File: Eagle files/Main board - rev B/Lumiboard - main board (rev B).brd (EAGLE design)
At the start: 49.7 x 42.2 mm, 29 parts, among them IC1 MCP1700, IC2 ULN2003AD, U1 ATMEGA328, U2 DX_BT_MODULE, Y1 8Mhz

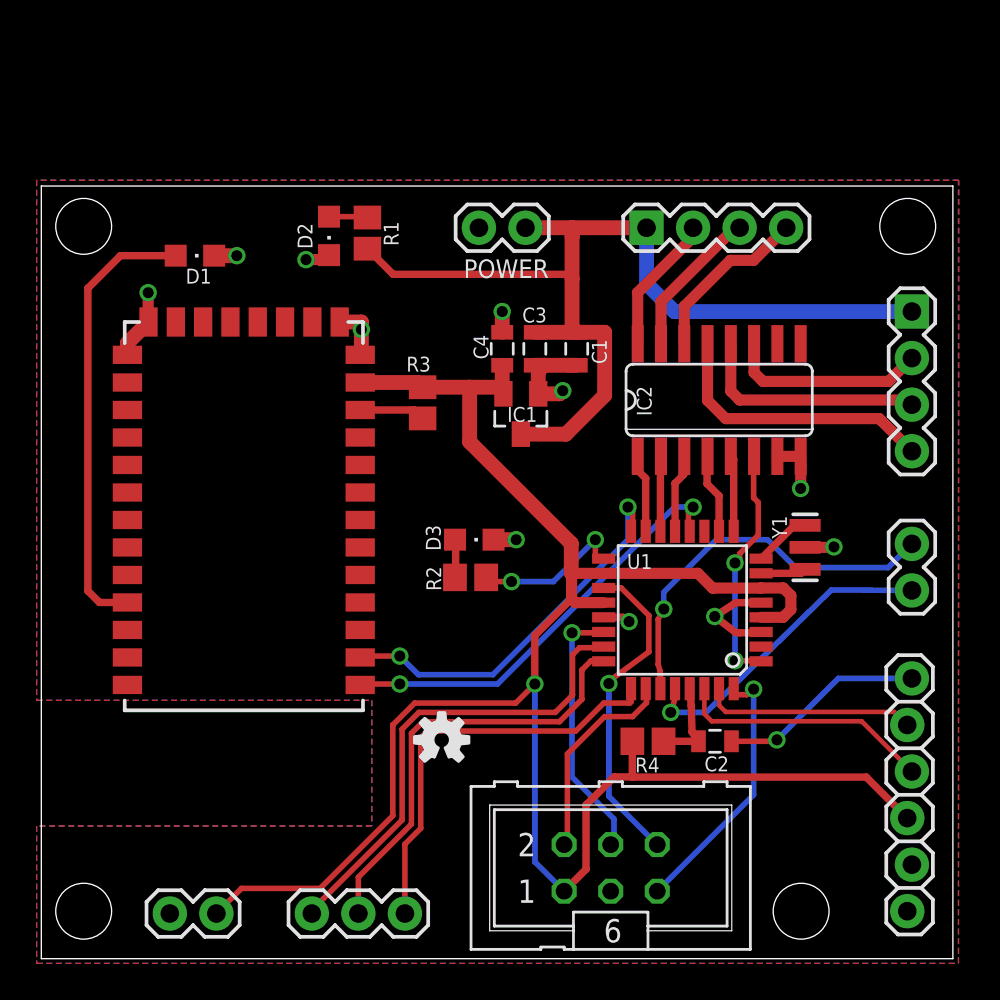
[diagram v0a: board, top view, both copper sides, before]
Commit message: New BOM, board files and readme
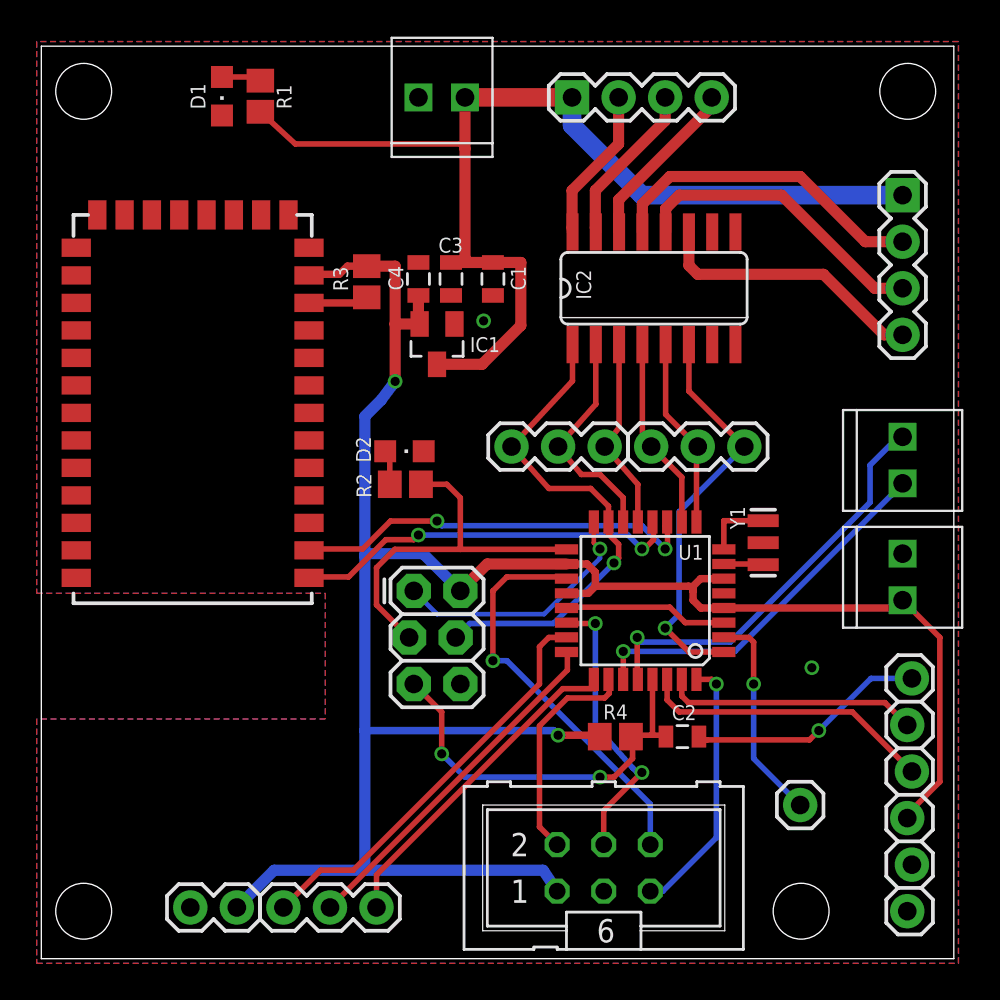
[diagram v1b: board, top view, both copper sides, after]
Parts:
- removed D3: DEBUG, led:CHIPLED_0805
- removed I2C: JP3, SparkFun:1X02
- removed LED1: JP5, SparkFun-Connectors:1X04
- removed LED2: JP6, SparkFun-Connectors:1X04
- removed POTSIN: JP4, SparkFun:1X03
- removed POTSPWR: JP2, SparkFun:1X02
- removed POWER: JP1, SparkFun:1X02
- removed U$1: (no value), SparkFun:OSHW-LOGO-S
- added H1, H2, H4: STAND-OFFTIGHT, SparkFun:STAND-OFF-TIGHT
- added J1: AVR_SPI_PRG_62X3_LOCK, SparkFun-Connectors:2X3_LOCK
- added J4: I2CDATA, SparkFun-Connectors:1X02_2.54_SCREWTERM
- added JP1: POWER, SparkFun-Connectors:1X02_2.54_SCREWTERM
- added JP10, JP11: (no value), SparkFun-Connectors:1X03
- added JP6: FTDI, SparkFun:1X06_LOCK
- added JP8: POTSIN, SparkFun:1X03
- added JP9: POTPOWER, SparkFun:1X02
- added LOGO1: OSHW-LOGOL, SparkFun-Aesthetics:OSHW-LOGO-L
- C2: value .1uF -> 1uF
- D1: value BLUE -> GREEN
- D2: value GREEN -> DEBUG
- JP2: value STAND-OFFTIGHT -> RGBLED1; device SparkFun:STAND-OFF-TIGHT -> SparkFun-Connectors:1X04
- JP3: value STAND-OFFTIGHT -> RGBLED2; device SparkFun:STAND-OFF-TIGHT -> SparkFun-Connectors:1X04
- JP5: value STAND-OFFTIGHT -> 3V3OUT; device SparkFun:STAND-OFF-TIGHT -> SparkFun-Connectors:1X02_2.54_SCREWTERM
- JP7: value FTDI -> D4; device SparkFun:1X06_LOCK -> SparkFun-Connectors:1X01
- SV1: value (none) -> SENSORS
- moved JP5 47.8 mm to (47.0, 19.6), turned to 90 degrees
- moved JP2 44.7 mm to (47.0, 41.7), turned to 270 degrees
- moved JP3 19.6 mm to (29.0, 47.0)
- moved D2 12.4 mm to (19.8, 27.7), turned to 270 degrees
- moved R1 9.48 mm to (12.0, 47.1)
- moved JP7 9.21 mm to (41.4, 8.38), turned to 0 degrees
- moved D1 8.82 mm to (9.86, 47.1), turned to 180 degrees
- moved R3 7.27 mm to (17.8, 36.9)
- moved IC2 7.06 mm to (33.4, 36.6)
- moved U2 6.48 mm to (8.26, 27.1)
- moved R2 6.20 mm to (19.9, 25.9)
- moved C1 5.95 mm to (24.6, 37.1)
- moved C3 5.95 mm to (22.4, 37.1)
- moved C4 5.95 mm to (20.6, 37.1)
- moved IC1 5.95 mm to (21.6, 33.5)
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- renumbered JP4 to H3
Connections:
- net N$11 renamed BTRESET
- removed net N$12: POTSIN.3, U1.25
- removed net N$14: IC2.13, LED1.4
- removed net N$15: IC2.12, LED1.3
- removed net N$16: IC2.11, LED1.2
- removed net N$2: D1.A, U2.P$31
- removed net N$20: POTSIN.2, U1.24
- removed net N$22: POTSIN.1, U1.23
- new net MISO: J1.1, U1.16
- new net N$6: IC2.12, JP2.3
- new net PD4: JP7.1, U1.2
- new net POT1: JP8.1, U1.23
- new net POT2: JP8.2, U1.24
- new net POT3: JP8.3, U1.25
- new net RESET: C2.2, J1.5, R4.1, U1.29
- new net SCK: J1.3, R2.2, U1.17
- net +5V: now also JP1.P2, JP2.1, JP3.1; no longer LED1.1, LED2.1, POWER.2
- net 3.3V: now also J1.2, JP5.P2, JP6.4, JP9.2; no longer JP7.4, POTSPWR.2
- net B1: now also JP11.3
- net B2: now also JP10.3
- net BRX: now also U1.11; no longer U1.16
- net DTR: now also JP6.1; no longer JP7.1
- net G1: now also JP11.2
- net G2: now also JP10.2
- net GND: now also J1.6, JP1.P1, JP5.P1, JP6.5, JP6.6, JP9.1; no longer D3.C, JP7.5, JP7.6, POTSPWR.1, POWER.1
- net N$1: now also JP3.2; no longer LED2.2
- net N$10: now also IC2.11, JP2.4; no longer C2.2, R4.1, U1.29
- net N$13: now also D2.A; no longer D3.A
- net N$3: now also JP3.3; no longer LED2.3
- net N$4: now also IC2.13, JP2.2; no longer R2.2, U1.17
- net N$5: now also JP3.4; no longer LED2.4
- net N$9: now also D1.A; no longer D2.A
- net R1: now also J1.4, JP11.1
- net R2: now also JP10.1
- net RXI: now also JP6.2; no longer JP7.2
- net SCL: now also J4.P1; no longer I2C.1
- net SDA: now also J4.P2; no longer I2C.2
- net TXO: now also JP6.3; no longer JP7.3
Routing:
- net N$22: track 26.3 -> 0.00 mm
- net N$2: track 24.5 -> 0.00 mm
- net N$20: track 24.1 -> 0.00 mm
- net R1: track 4.29 -> 27.3 mm, vias 0 -> 1
- net N$12: track 23.0 -> 0.00 mm
- net POT1: track 0.00 -> 22.7 mm
- net RESET: track 0.00 -> 22.6 mm, vias 0 -> 2
- net GND: track 29.6 -> 8.95 mm, vias 11 -> 2
- net SCK: track 0.00 -> 20.6 mm
- net POT2: track 0.00 -> 19.3 mm
- net POT3: track 0.00 -> 18.5 mm
- net N$6: track 0.00 -> 16.6 mm
- net N$14: track 15.4 -> 0.00 mm
- net 3.3V: track 109.3 -> 123.5 mm, vias 1 -> 2
- net MISO: track 0.00 -> 14.1 mm, vias 0 -> 1
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- added copper zone on layer 1, net GND
- removed copper zone on layer 1, net N$6
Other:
- board size 49.7 x 42.2 mm -> 49.8 x 49.8 mm
- board text added: "(RAW PWM)"
- board text added: "-"
- board text added: "10"
- board text added: "11"
- board text added: "3"
- board text added: "3V3"
- board text added: "5"
- board text added: "6"
- board text added: "9"
- board text added: "A3"
- board text added: "A6"
- board text added: "A7"
- board text added: "CTS"
- board text added: "Common anode LEDs only!"
- board text added: "D2"
- board text added: "DTR"
- board text added: "Designed by Jason Webb"
- board text added: "Each LED pin can sink up to 500mA"
- board text added: "IN"
- board text added: "MISO"
- board text added: "MOSI"
- board text added: "Power breakout"
- board text added: "REV B"
- board text added: "RST"
- board text added: "RXI"
- board text added: "SCK"
- board text added: "TXO"
- board text added: "http://jason-webb.info"
- board text removed: "ATMEGA328"
- board text removed: "Jason Webb"
- board text removed: "LUMIBOARD"
- board text removed: "Lead engineer + designe"
- board text removed: "MAIN BOARD"
- board text removed: "PCB design help from Stew Koch"
- board text removed: "REV A"
